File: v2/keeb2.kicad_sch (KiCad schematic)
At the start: 30 parts, among them J1 AVR-ISP-6, SW2 SW_Push_Reset, U1 ATmega32U4-A, Y1 XTAL

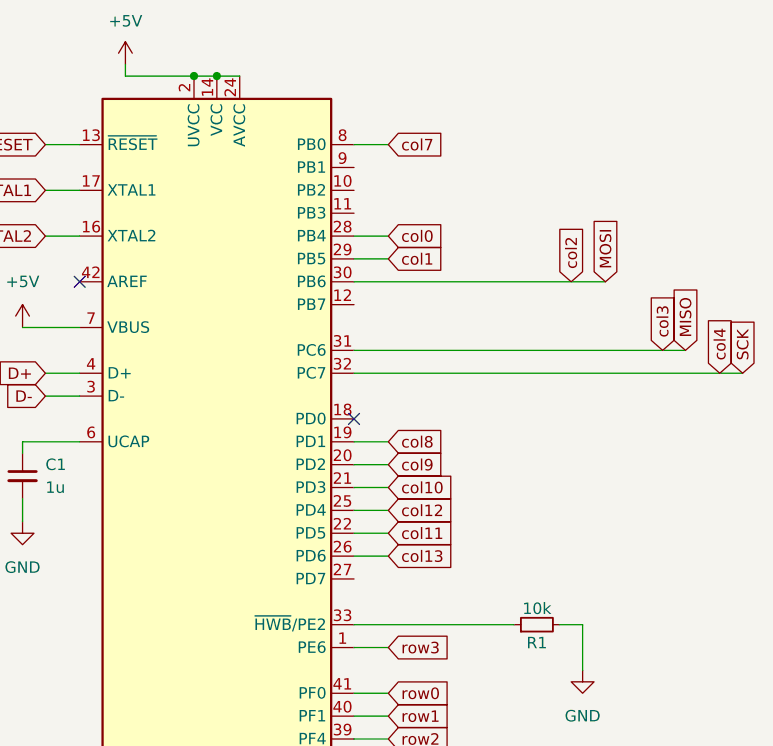
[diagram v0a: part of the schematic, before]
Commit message: Finished routing
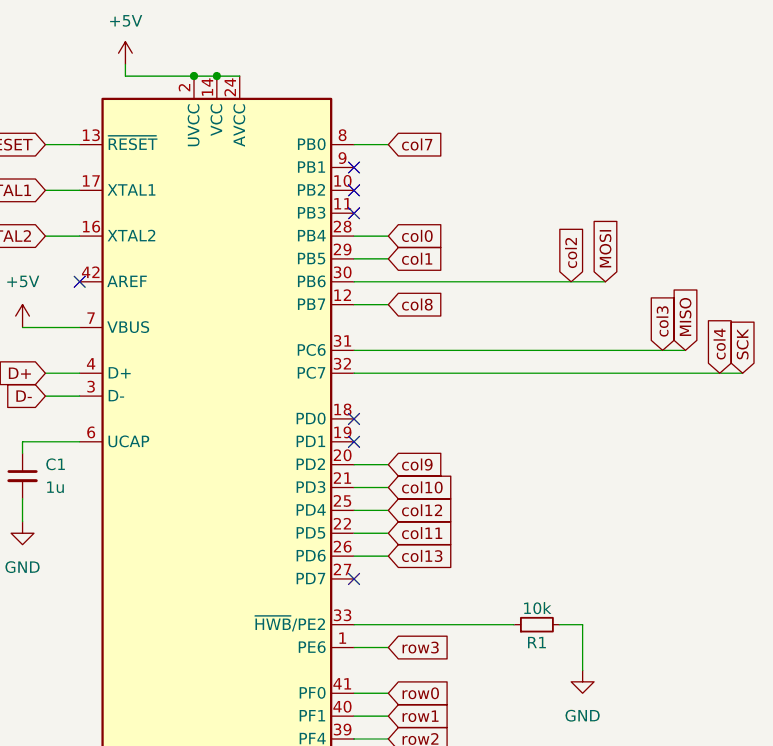
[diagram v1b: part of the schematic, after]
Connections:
- net col8: now also U1.12 (PB7); no longer U1.19 (PD1)
- no-connect marks 4 -> 9
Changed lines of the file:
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@@
+	)
+	(no_connect
+		(at 210.82 49.53)
 	)
 	(no_connect
@@
 	)
 	(no_connect
+		(at 210.82 80.01)
+	)
+	(no_connect
+		(at 210.82 95.25)
+	)
+	(no_connect
+		(at 210.82 52.07)
+	)
+	(no_connect
 		(at 39.37 71.12)
 	)
+	(no_connect
+		(at 210.82 54.61)
+	)
 	(wire
 		(pts
@@
 	(wire
 		(pts
+			(xy 210.82 64.77) (xy 214.63 64.77)
+		)
+		(stroke
+			(width 0)
+			(type default)
+		)
+	)
+	(wire
+		(pts
 			(xy 193.04 134.62) (xy 195.58 134.62)
 		)
@@
 	(wire
 		(pts
-			(xy 210.82 80.01) (xy 214.63 80.01)
-		)
-		(stroke
-			(width 0)
-			(type default)
-		)
-	)
-	(wire
-		(pts
 			(xy 45.72 78.74) (xy 45.72 83.82)
 		)
@@
 		)
 	)
+	(global_label "col8"
+		(shape input)
+		(at 214.63 64.77 0)
+		(fields_autoplaced yes)
+		(effects
+			(font
+				(size 1.27 1.27)
+			)
+			(justify left)
+		)
+		(property "Intersheetrefs" "${INTERSHEET_REFS}"
+			(at 221.7275 64.77 0)
+			(effects
+				(font
+					(size 1.27 1.27)
+				)
+				(justify left)
+				(hide yes)
+			)
+		)
+	)
 	(global_label "col13"
 		(shape input)
@@
 				(hide yes)
 			)
-		)
-	)
-	(global_label "col8"
-		(shape input)
-		(at 214.63 80.01 0)
-		(fields_autoplaced yes)
-		(effects
-			(font
-				(size 1.27 1.27)
-			)
-			(justify left)
-		)
-		(property "Intersheetrefs" "${INTERSHEET_REFS}"
-			(at 221.7275 80.01 0)
-			(effects
-				(font
-					(size 1.27 1.27)
-				)
-				(justify left)
-				(hide yes)
-			)
